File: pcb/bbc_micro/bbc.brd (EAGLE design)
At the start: 43 x 30 mm, 25 parts, among them U2 LM2776

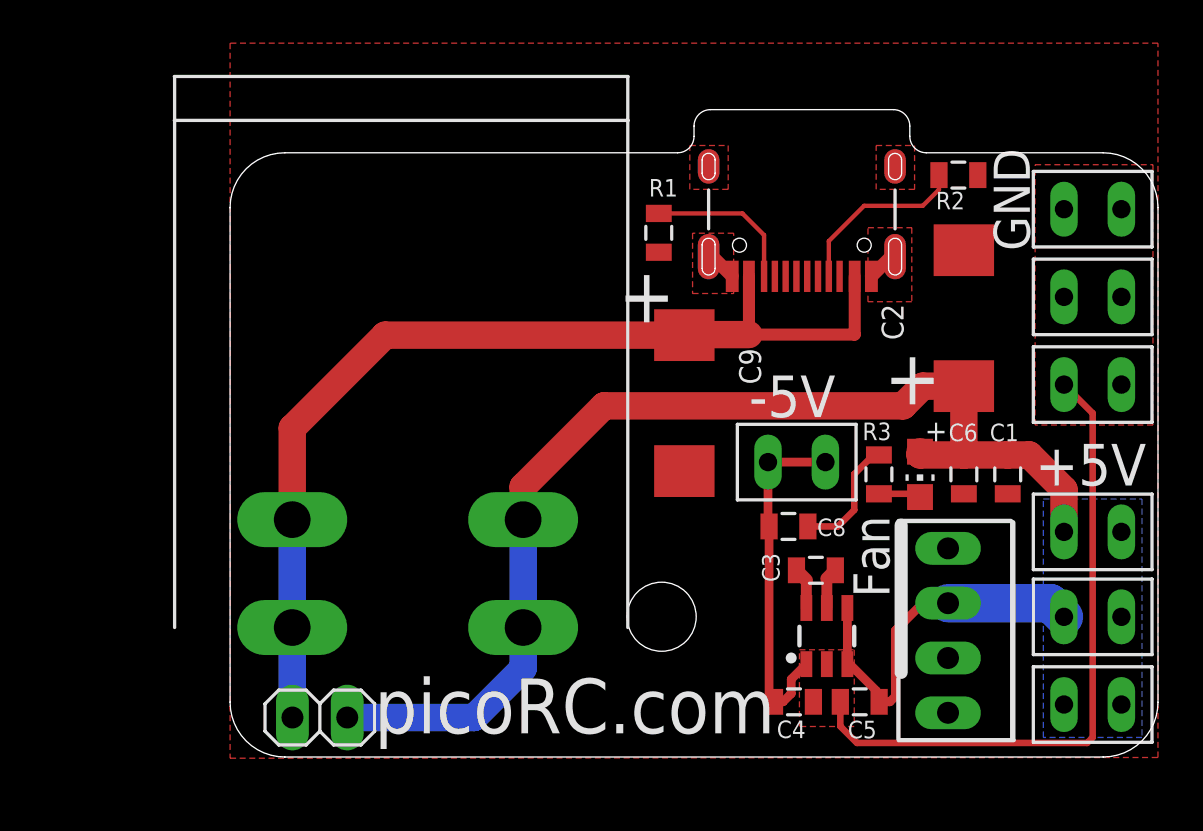
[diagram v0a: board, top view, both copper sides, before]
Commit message: minor adjustment before production
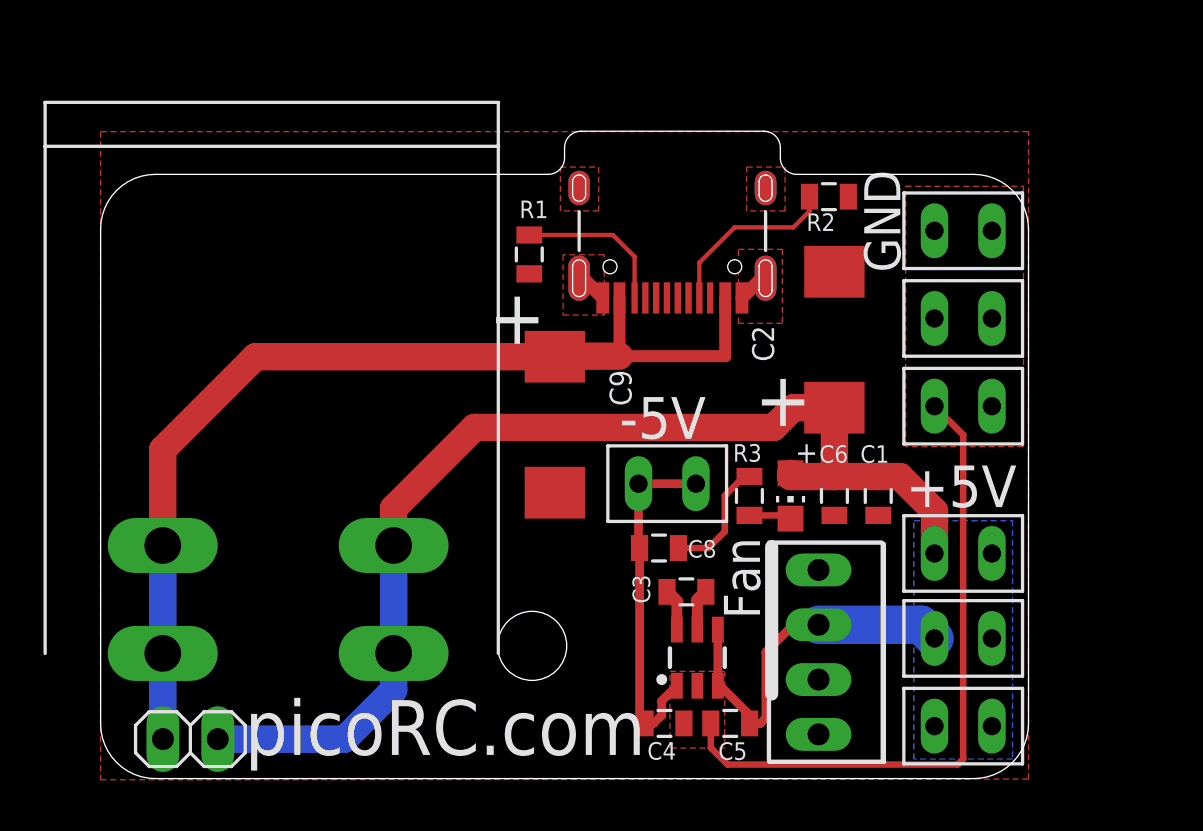
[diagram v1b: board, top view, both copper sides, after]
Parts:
- moved U$4 6.15 mm to (20.0, 6.15)
- moved U$3 6.12 mm to (7.93, 5.80)
- moved C5 6.08 mm to (29.2, 2.56)
- moved J4 6.08 mm to (26.5, 22.3)
- moved U$5 6.08 mm to (26.3, 13.7)
- moved JP1 6.08 mm to (4.16, 1.83)
- moved C1 6.08 mm to (36.0, 13.1)
- moved C2 6.08 mm to (34.0, 20.3)
- moved C3 6.08 mm to (27.1, 8.65)
- moved C4 6.08 mm to (26.1, 2.56)
- moved C6 6.08 mm to (34.0, 13.1)
- moved C8 6.08 mm to (25.9, 10.7)
- moved C9 6.08 mm to (21.1, 16.4)
- moved JP3 6.08 mm to (33.3, 5.86)
- moved LED3 6.08 mm to (32.0, 13.1)
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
